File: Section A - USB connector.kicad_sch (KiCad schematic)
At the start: 3 parts, among them J2 USB4135-GF-A_REVA

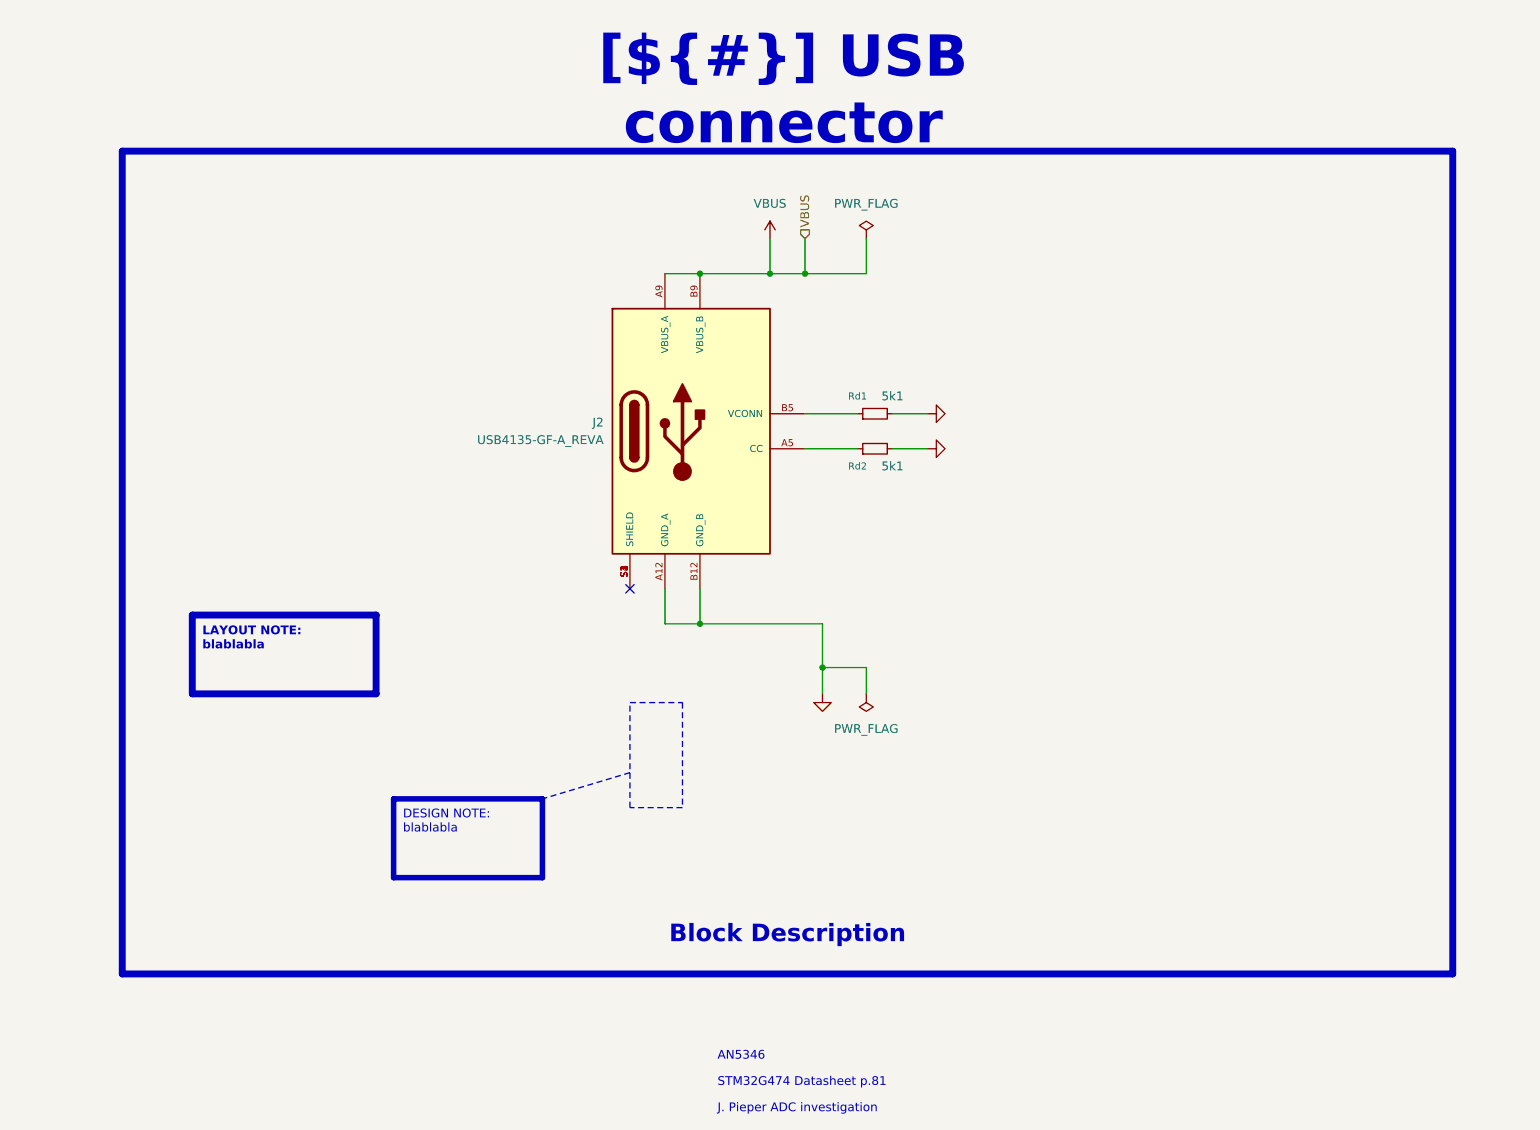
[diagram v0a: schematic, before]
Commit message: touch pad library creation
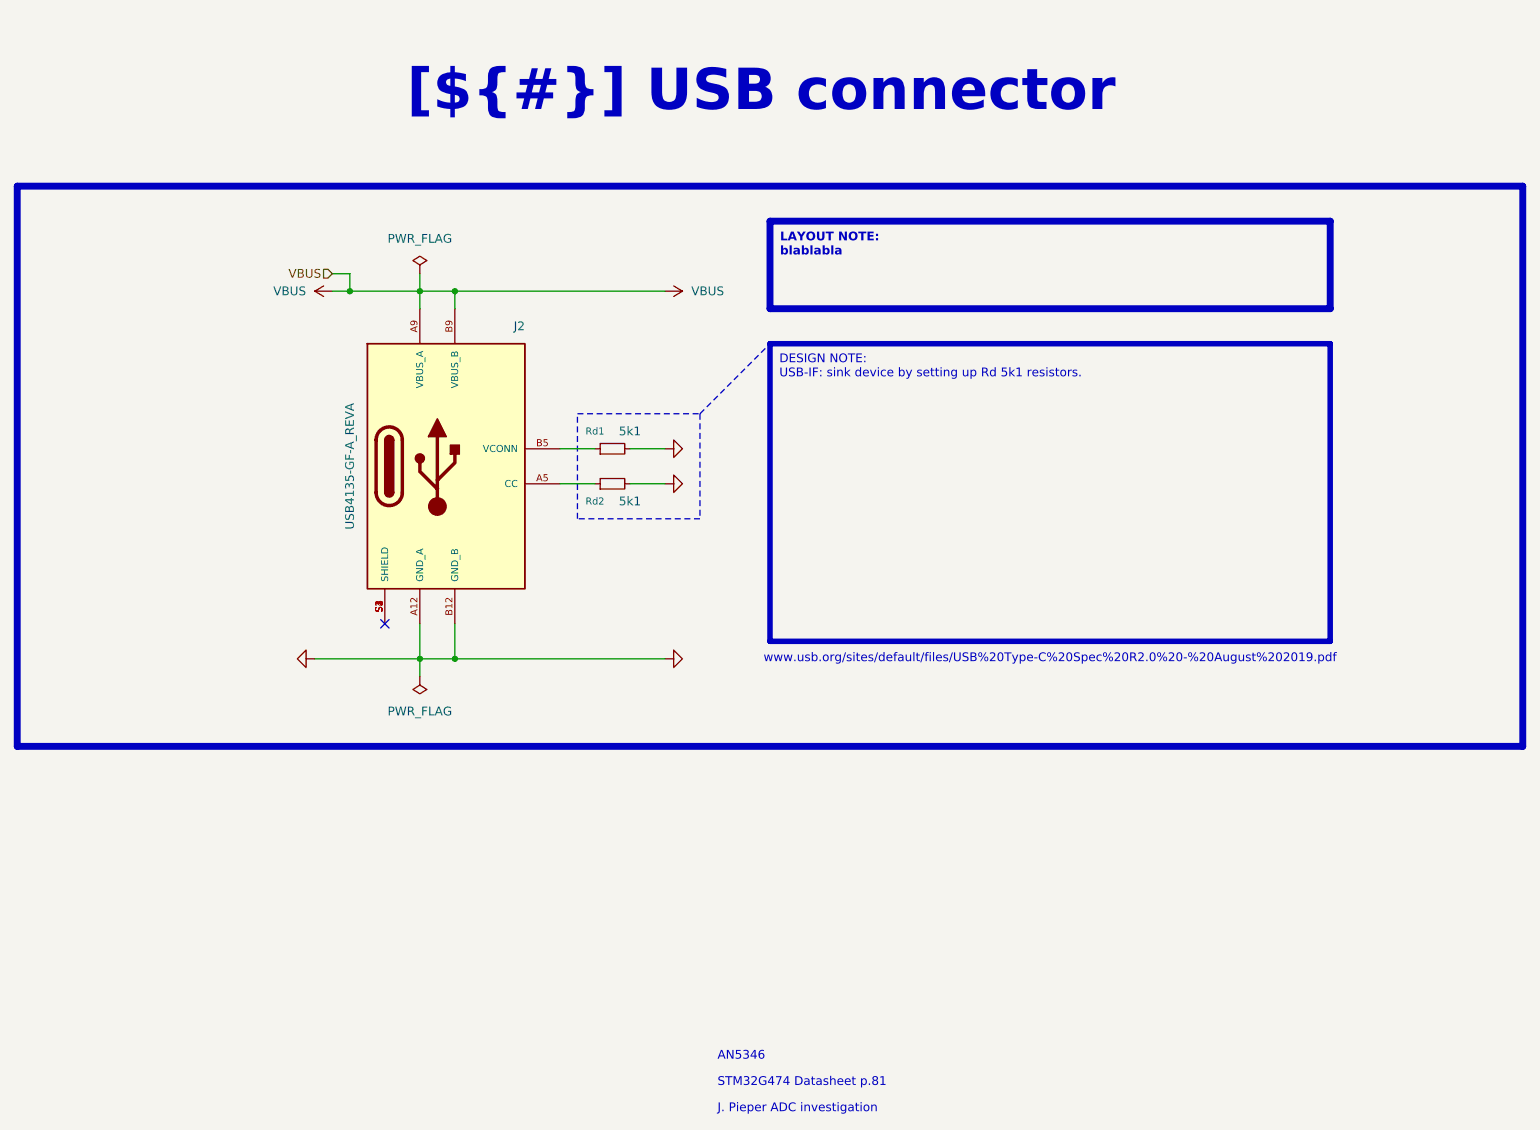
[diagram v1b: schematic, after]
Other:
- note added: "www.usb.org/sites/default/files/USB%20Type-C%20Spec%20R2.0%20-%20August%202019.pdf"
- moved on the sheet: J2, Rd1, Rd2
